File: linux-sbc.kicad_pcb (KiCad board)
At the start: 8 copper layers, 524 parts, among them J1001 7499010121A, J101 Mini-fit Jr 5569, J1101 DM3AT-SF-PEJM5, J1201 PH1-08-UA, J1202 EMI shield frame, J1203 FH12A-40S-0.5SH(55), J1301 SMA RF2-04, J201 61300211121, J202 61300211121, J203 61300211121, J204 61300211121, J205 61300211121, J206 61300211121, J207 61300211121, J208 61300211121, J301 61300211121, J302 61300211121, J303 EMI shield frame, J401 Conn_01x04, J402 EMI shield frame, J701 USB4105-GF-A, J702 TC2050-NL, J901 AU-Y1008-2-BLK, J902 AU-Y1008-2-BLK, Q201 DMPH4029LFGQ, Q202 DMPH4029LFGQ, Q203 DMN65D8L, Q204 DMPH4029LFGQ, Q205 DMPH4029LFGQ, SW501 JS202011CQN, U1001 LAN8742A-CZ-TR, U1201 TCA9554PW, U1202 AP5725FDCG-7, U1301 LBEE5KL1YN-814, U201 LM4040-5.0, U202 TL331, U203 OPA197, U204 LM4040-5.0, U205 TL331, U206 LM4040-5.0, U207 TL331, U301 AP64500SP-13, U302 AP64500SP-13, U401 STPMIC1DPQR, U501 STM32MP135FAE7, U701 FT231XQ-R, U702 TCA9554PW, U801 MT41K256M16TW, U901 USB2514B/M2, U902 AP22966DC8-7, U903 AP22966DC8-7, Y501 32.768 kHz, Y502 24 MHz, Y901 24 MHz

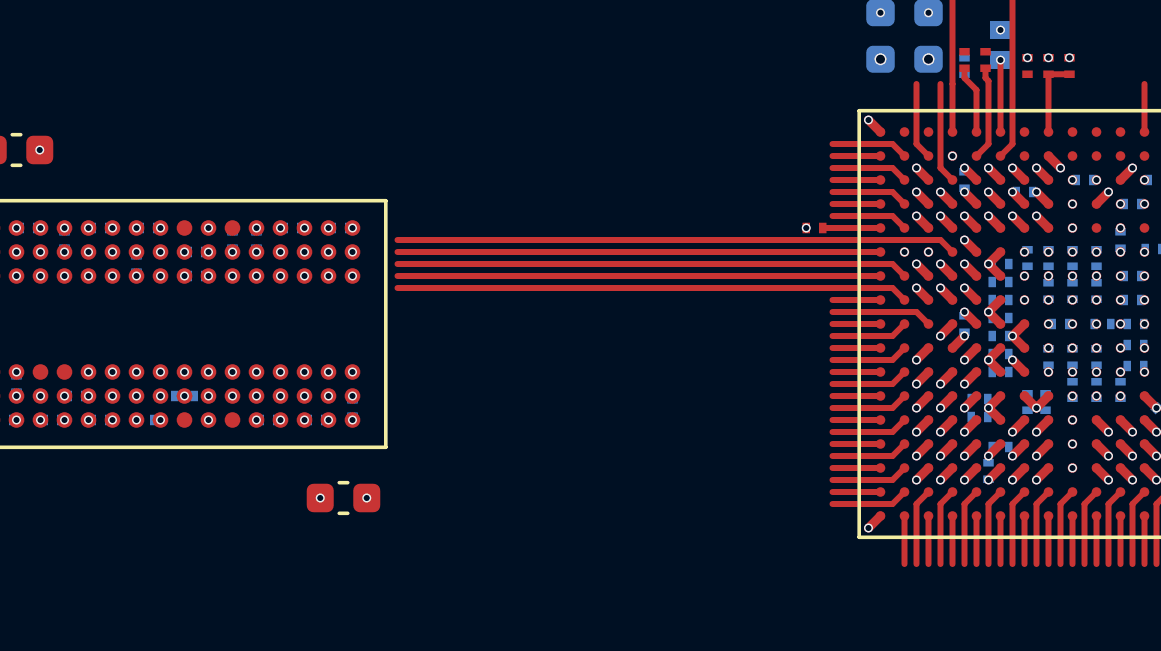
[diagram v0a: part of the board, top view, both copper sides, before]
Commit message: DDR AC first iteration
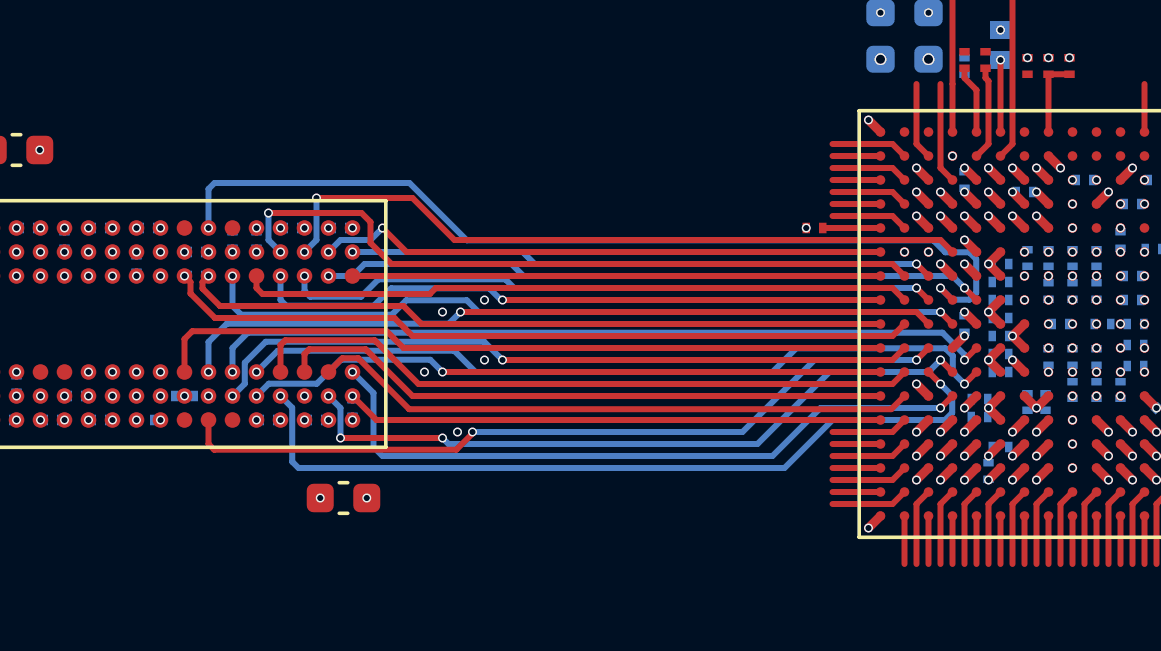
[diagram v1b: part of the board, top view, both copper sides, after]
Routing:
- net /DDR/DDR.CKE: track 0.57 -> 31.2 mm
- net /DDR/DDR.A3: track 0.57 -> 26.9 mm
- net /DDR/DDR.WE_N: track 0.57 -> 26.5 mm
- net /DDR/DDR.ODT: track 0.57 -> 26.3 mm
- net /DDR/DDR.BA2: track 0.57 -> 25.9 mm
- net /DDR/DDR.A10: track 0.57 -> 25.6 mm
- net /DDR/DDR.RAS_N: track 1.60 -> 24.6 mm, vias 1 -> 0
- net /DDR/DDR.A7: track 0.57 -> 23.4 mm, vias 2 -> 4
- net /DDR/DDR.CLK_P: track 2.57 -> 25.2 mm
- net /DDR/DDR.A13: track 0.57 -> 23.0 mm
- net /DDR/DDR.CAS_N: track 3.37 -> 25.6 mm, vias 1 -> 2
- net /DDR/DDR.CLK_N: track 1.60 -> 23.6 mm
- net /DDR/DDR.A11: track 0.57 -> 22.3 mm
- net /DDR/DDR.CS_N: track 2.57 -> 24.0 mm, vias 1 -> 2
- net /DDR/DDR.A1: track 0.57 -> 21.9 mm
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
